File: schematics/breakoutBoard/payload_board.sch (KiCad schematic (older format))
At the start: 7 parts, among them P1 CONN_02X50, P2 CONN_02X50, P3 CONN_02X50, P4 CONN_02X50, U1 breakout_carrier

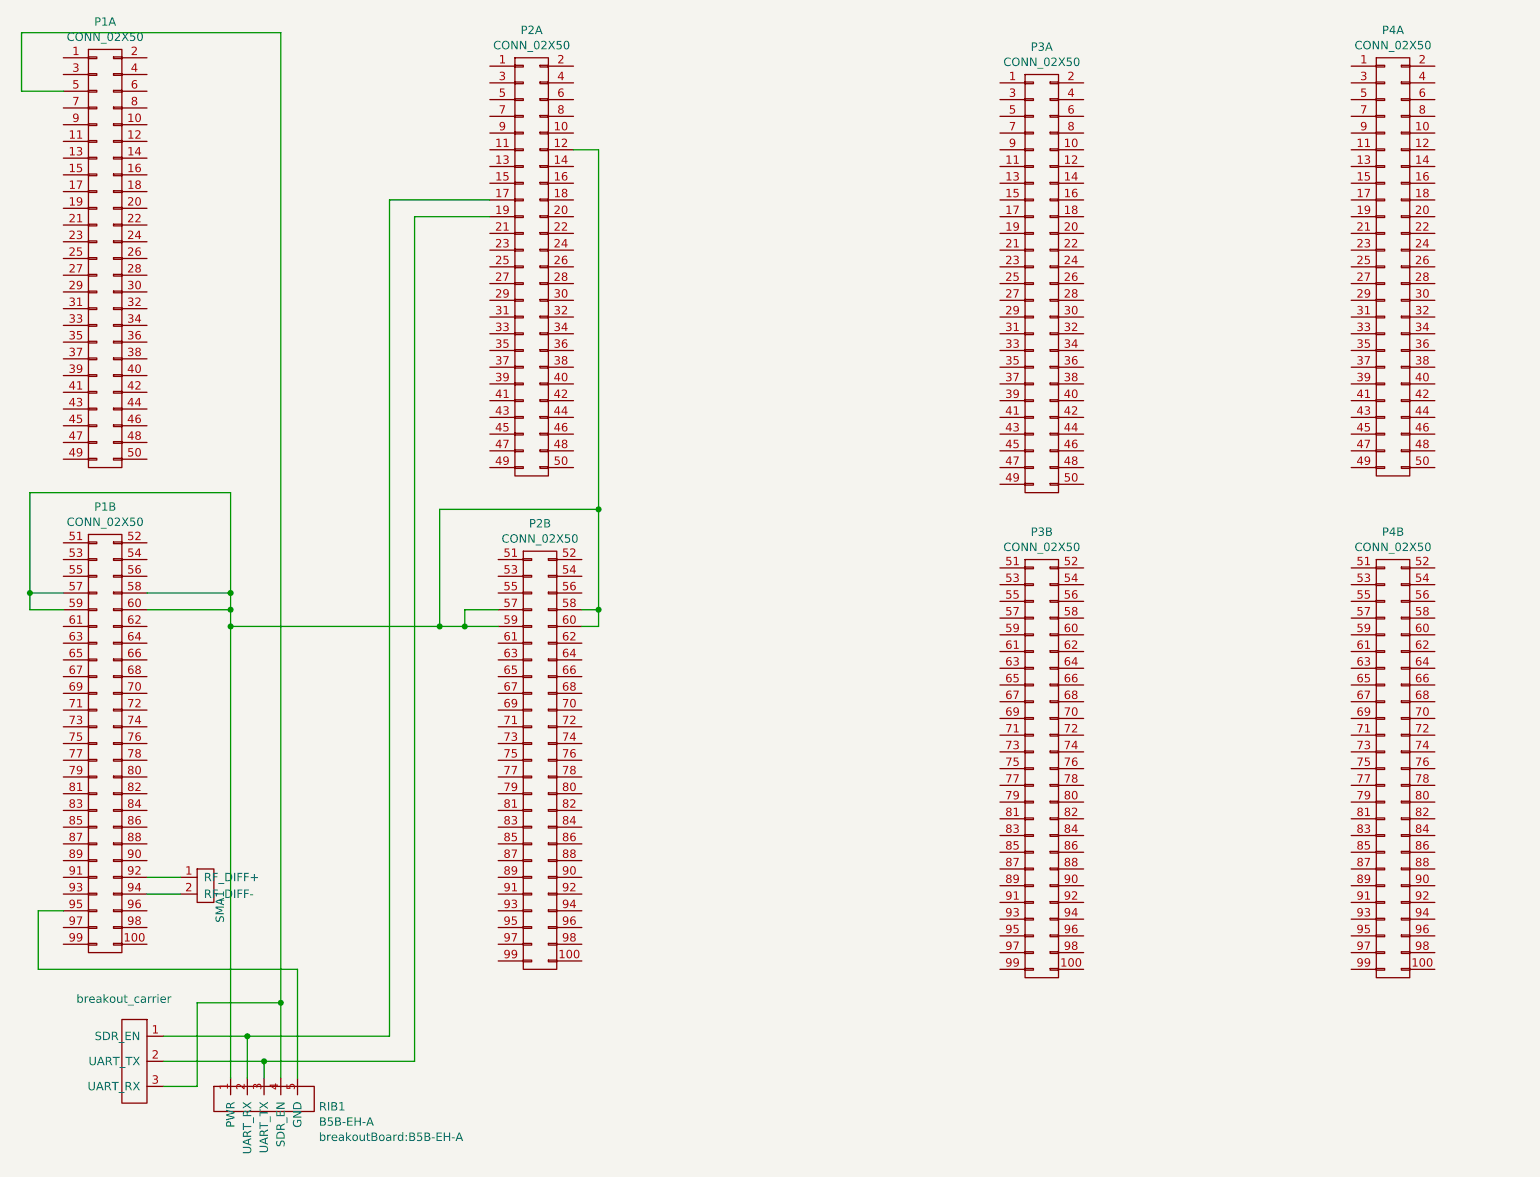
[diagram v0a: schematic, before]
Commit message: 'final' push
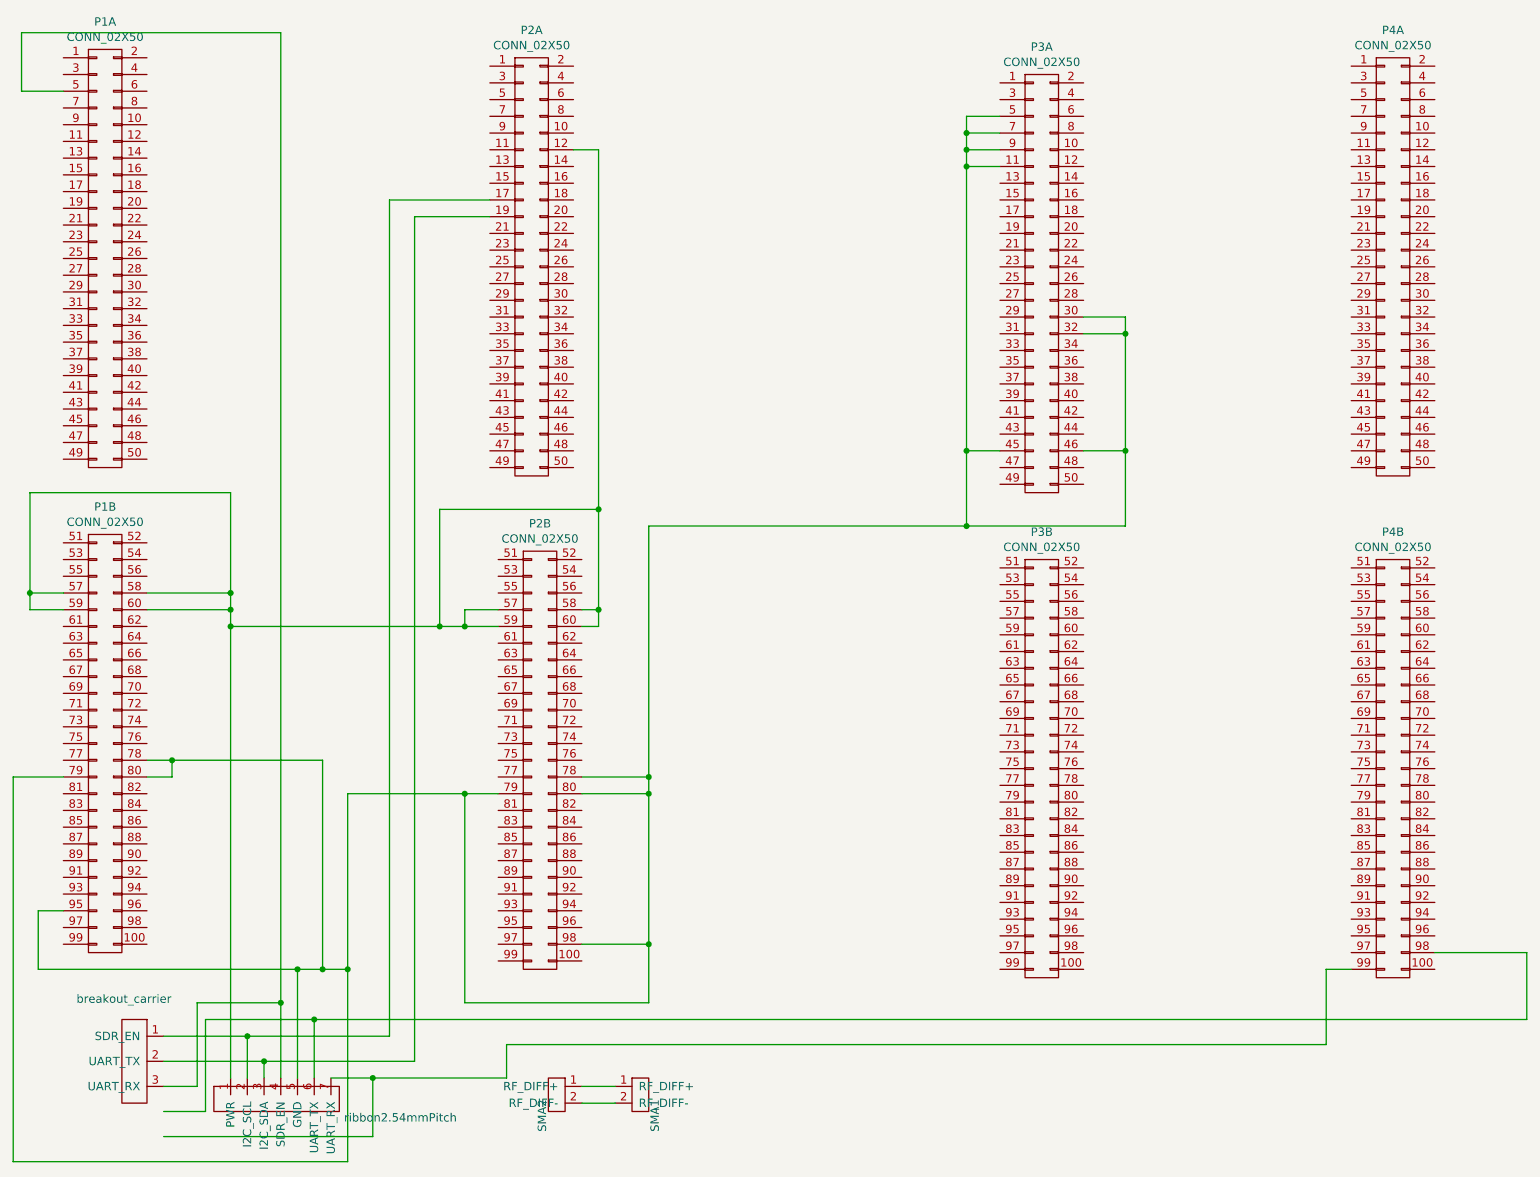
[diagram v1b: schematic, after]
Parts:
- removed RIB1: B5B-EH-A, breakoutBoard:B5B-EH-A, symbol payload_board-rescue:B5B-EH-A
- added SMA2: Molex-MMCX-SMD, breakoutBoard:Molex MMCX SMD 50Ohm, symbol payload_board-rescue:Molex-MMCX-SMD
- added e1: ribbon2.54mmPitch, breakoutBoard:ribbon2.5mmPitch, symbol payload_board-rescue:ribbon2.54mmPitch
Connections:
- net at P2.17 (P17), U1.1 (SDR_EN): now also e1.2 (I2C_SCL)
- net at P2.19 (P19), U1.2 (UART_TX): now also e1.3 (I2C_SDA)
- net at P1.5 (P5), U1.3 (UART_RX): now also e1.4 (SDR_EN)
- net at P1.57 (P57), P1.58 (P58), P1.59 (P59)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: now also e1.1 (PWR)
- net at P3.11 (P11): now also P1.78 (P78), P1.79 (P79), P1.80 (P80), P1.95 (P95), P2.78 (P78), P2.79 (P79), P2.80 (P80), P2.98 (P98), P3.30 (P30), P3.32 (P32), P3.45 (P45), P3.46 (P46), P3.5 (P5), P3.7 (P7), P3.9 (P9), e1.5 (GND)
- net at P1.92 (P92): no longer SMA1.1 (RF_DIFF+)
- net at P1.94 (P94): no longer SMA1.2 (RF_DIFF-)
- net at P4.98 (P98): now also e1.6 (UART_TX)
- net at P4.99 (P99): now also e1.7 (UART_RX)
- new net: SMA1.1 (RF_DIFF+), SMA2.1 (RF_DIFF+)
- new net: SMA1.2 (RF_DIFF-), SMA2.2 (RF_DIFF-)
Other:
- moved on the sheet: SMA1
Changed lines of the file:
@@
-	1    0    0    -1
-$EndComp
-$Comp
-L payload_board-rescue:B5B-EH-A RIB1
-U 1 1 5CCD2E38
-P 2800 7150
-F 0 "RIB1" H 3078 7079 50  0000 L CNN
-F 1 "B5B-EH-A" H 3078 6988 50  0000 L CNN
-F 2 "breakoutBoard:B5B-EH-A" H 3078 6897 50  0000 L CNN
-F 3 "" H 2750 7250 50  0001 C CNN
-	1    2800 7150
 	1    0    0    -1
 $EndComp
@@
 L payload_board-rescue:Molex-MMCX-SMD SMA1
 U 1 1 5CCDD268
-P 2350 5850
-F 0 "SMA1" H 2428 5713 50  0000 L CNN
-F 1 "Molex-MMCX-SMD" H 2350 6100 50  0001 C CNN
-F 2 "breakoutBoard:Molex MMCX SMD 50Ohm" H 2350 5850 50  0001 C CNN
-F 3 "" H 2350 5850 50  0001 C CNN
-	1    2350 5850
+P 4950 7100
+F 0 "SMA1" H 5028 6963 50  0000 L CNN
+F 1 "Molex-MMCX-SMD" H 4950 7350 50  0001 C CNN
+F 2 "breakoutBoard:Molex MMCX SMD 50Ohm" H 4950 7100 50  0001 C CNN
+F 3 "" H 4950 7100 50  0001 C CNN
+	1    4950 7100
 	0    -1   1    0
 $EndComp
 Wire Wire Line
-	2250 5850 2050 5850
-Wire Wire Line
-	2250 5950 2050 5950
-Wire Wire Line
 	2950 7050 2950 6400
 Wire Wire Line
@@
 Wire Wire Line
 	1400 6400 2950 6400
+Wire Wire Line
+	2200 5150 2050 5150
+Wire Wire Line
+	2050 5250 2200 5250
+Wire Wire Line
+	2200 5250 2200 5150
+Wire Wire Line
+	1550 5250 1250 5250
+Wire Wire Line
+	1250 5250 1250 7550
+Wire Wire Line
+	1250 7550 3250 7550
+Wire Wire Line
+	3250 7550 3250 6400
+Wire Wire Line
+	3250 6400 3100 6400
+Connection ~ 2950 6400
+Wire Wire Line
+	3250 6400 3250 5350
+Wire Wire Line
+	3250 5350 3950 5350
+Connection ~ 3250 6400
+Wire Wire Line
+	4650 5250 5050 5250
+Wire Wire Line
+	5050 5250 5050 5350
+Wire Wire Line
+	5050 6600 3950 6600
+Wire Wire Line
+	3950 6600 3950 5350
+Connection ~ 3950 5350
+Wire Wire Line
+	3950 5350 4150 5350
+Wire Wire Line
+	4650 5350 5050 5350
+Connection ~ 5050 5350
+Wire Wire Line
+	5050 5350 5050 6250
+Wire Wire Line
+	4650 6250 5050 6250
+Connection ~ 5050 6250
+Wire Wire Line
+	5050 6250 5050 6600
+Wire Wire Line
+	7650 3300 7900 3300
+Wire Wire Line
+	7900 3300 7900 3750
+Wire Wire Line
+	7900 3750 6950 3750
+Wire Wire Line
+	5050 3750 5050 5250
+Connection ~ 5050 5250
+Wire Wire Line
+	7150 3300 6950 3300
+Connection ~ 6950 3750
+Wire Wire Line
+	6950 3750 5050 3750
+Wire Wire Line
+	7650 2500 7900 2500
+Wire Wire Line
+	7900 2500 7900 2600
+Connection ~ 7900 3300
+Wire Wire Line
+	7650 2600 7900 2600
+Connection ~ 7900 2600
+Wire Wire Line
+	7900 2600 7900 3300
+Wire Wire Line
+	7150 1300 6950 1300
+Wire Wire Line
+	6950 1300 6950 1400
+Connection ~ 6950 3300
+Wire Wire Line
+	6950 3300 6950 3750
+Wire Wire Line
+	7150 1400 6950 1400
+Connection ~ 6950 1400
+Wire Wire Line
+	6950 1400 6950 1500
+Wire Wire Line
+	7150 1500 6950 1500
+Connection ~ 6950 1500
+Wire Wire Line
+	6950 1500 6950 1600
+Wire Wire Line
+	7150 1600 6950 1600
+Connection ~ 6950 1600
+Wire Wire Line
+	6950 1600 6950 3300
+Wire Wire Line
+	2200 5150 3100 5150
+Wire Wire Line
+	3100 5150 3100 6400
+Connection ~ 2200 5150
+Connection ~ 3100 6400
+Wire Wire Line
+	3100 6400 2950 6400
+$Comp
+L payload_board-rescue:ribbon2.54mmPitch e1
+U 1 1 5CCBC1CC
+P 2700 7250
+F 0 "e1" H 3150 7250 50  0001 C CNN
+F 1 "ribbon2.54mmPitch" H 3228 7213 50  0000 L CNN
+F 2 "breakoutBoard:ribbon2.5mmPitch" H 3150 7250 50  0001 C CNN
+F 3 "" H 3150 7250 50  0001 C CNN
+	1    2700 7250
+	1    0    0    -1
+$EndComp
+$Comp
+L payload_board-rescue:Molex-MMCX-SMD SMA2
+U 1 1 5CCBDC56
+P 4550 7100
+F 0 "SMA2" H 4628 6963 50  0000 L CNN
+F 1 "Molex-MMCX-SMD" H 4550 7350 50  0001 C CNN
+F 2 "breakoutBoard:Molex MMCX SMD 50Ohm" H 4550 7100 50  0001 C CNN
+F 3 "" H 4550 7100 50  0001 C CNN
+	1    4550 7100
+	0    1    1    0
+$EndComp
+Wire Wire Line
+	4650 7100 4850 7100
+Wire Wire Line
+	4850 7200 4650 7200
+Wire Wire Line
+	9750 6300 10300 6300
+Wire Wire Line
+	10300 6300 10300 6700
+Wire Wire Line
+	10300 6700 3050 6700
+Wire Wire Line
+	3050 6700 3050 7050
+Wire Wire Line
+	3150 7050 3400 7050
+Wire Wire Line
+	4200 7050 4200 6850
+Wire Wire Line
+	4200 6850 9100 6850
+Wire Wire Line
+	9100 6850 9100 6400
+Wire Wire Line
+	9100 6400 9250 6400
+Wire Wire Line
+	2150 7250 2400 7250
+Wire Wire Line
+	2400 7250 2400 6700
+Wire Wire Line
+	2400 6700 3050 6700
+Connection ~ 3050 6700
+Wire Wire Line
+	3400 7050 3400 7400
+Wire Wire Line
+	3400 7400 2150 7400
+Connection ~ 3400 7050
+Wire Wire Line
+	3400 7050 4200 7050
 $EndSCHEMATC
